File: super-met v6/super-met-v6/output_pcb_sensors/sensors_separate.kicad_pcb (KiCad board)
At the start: 2 copper layers, 99.3 x 99.3 mm, 69 parts, among them J4 Conn_01x08, J5 Conn_01x08, J6 Conn_01x08, J7 Conn_01x04, J8 Conn_01x04, Q13 AO3400A, Q14 AO3400A, Q15 AO3400A, Q16 AO3400A, Q17 AO3400A, Q18 AO3400A, Q19 AO3400A, Q20 AO3400A, Q21 AO3400A, Q22 AO3400A, Q23 AO3400A, Q24 AO3400A, U15 MQ GENERIC BOARD SENSOR, U16 MQ GENERIC BOARD SENSOR, U17 MQ GENERIC BOARD SENSOR, U18 MQ GENERIC BOARD SENSOR, U19 MQ GENERIC BOARD SENSOR, U20 MQ GENERIC BOARD SENSOR, U21 MQ GENERIC BOARD SENSOR, U22 MQ GENERIC BOARD SENSOR, U23 AHT10 MODULE, U24 MQ GENERIC BOARD SENSOR, U25 MQ GENERIC BOARD SENSOR, U26 MICS-6814, U27 CCS811, U28 MS-1100

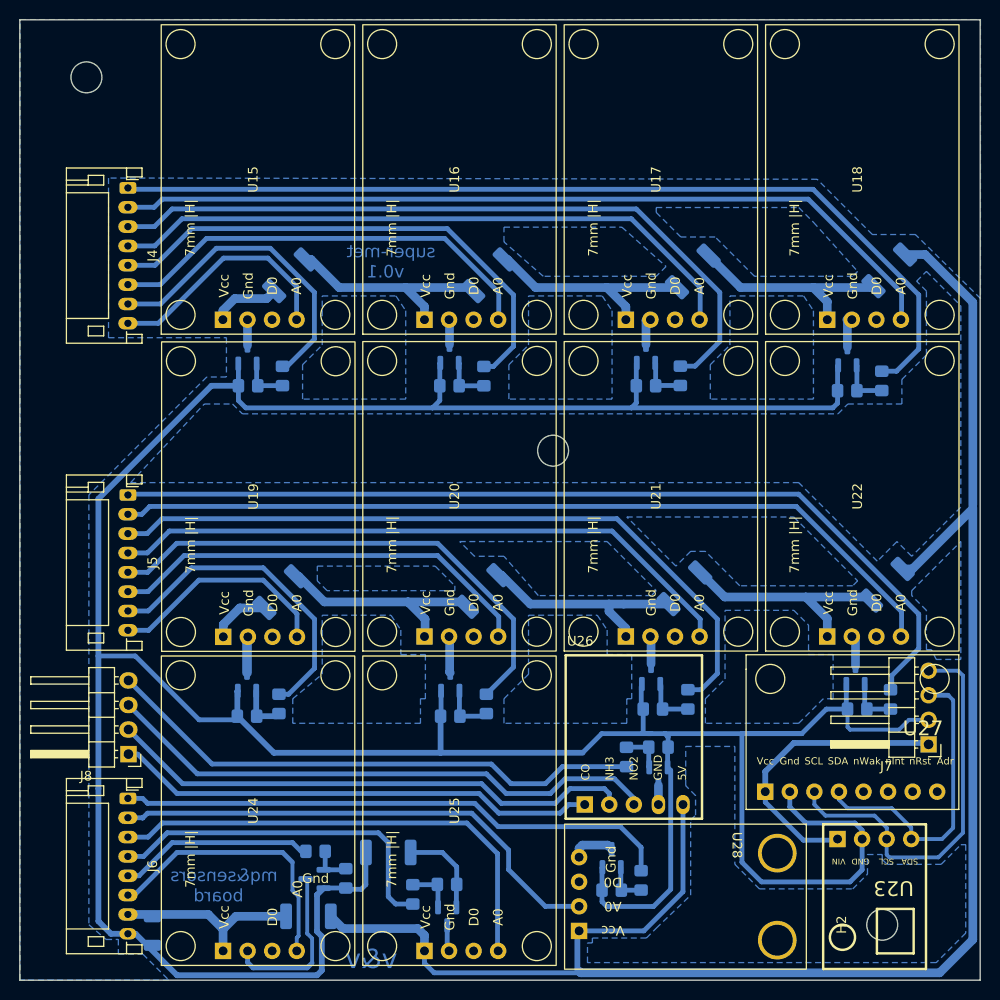
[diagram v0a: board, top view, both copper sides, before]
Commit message: preparing sensors board
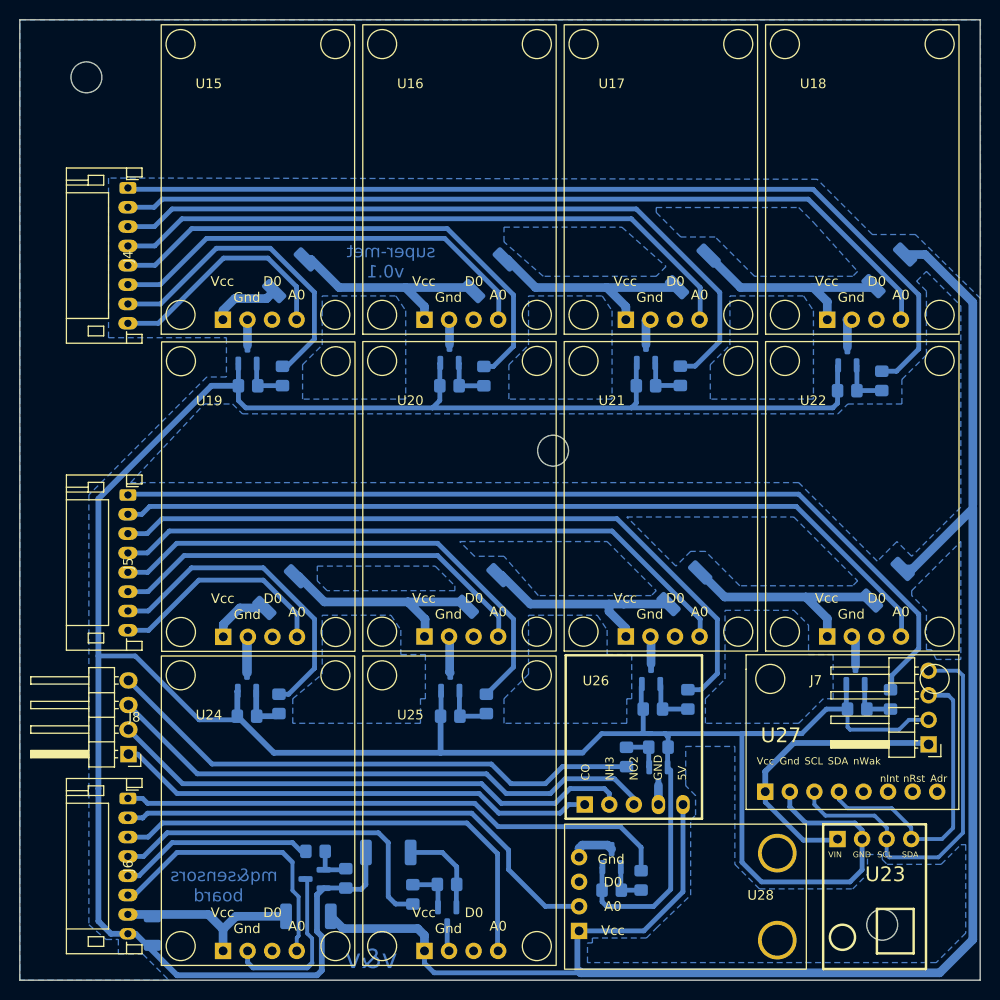
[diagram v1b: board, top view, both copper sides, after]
